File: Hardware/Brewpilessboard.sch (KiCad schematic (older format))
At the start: 10 parts, among them J1 Conn_01x01_Female, J2 Conn_01x01_Female, K1 2channelrelay, U1 ESP32_DevKit_V1_DOIT, U2 DS18B20, U3 DS18B20

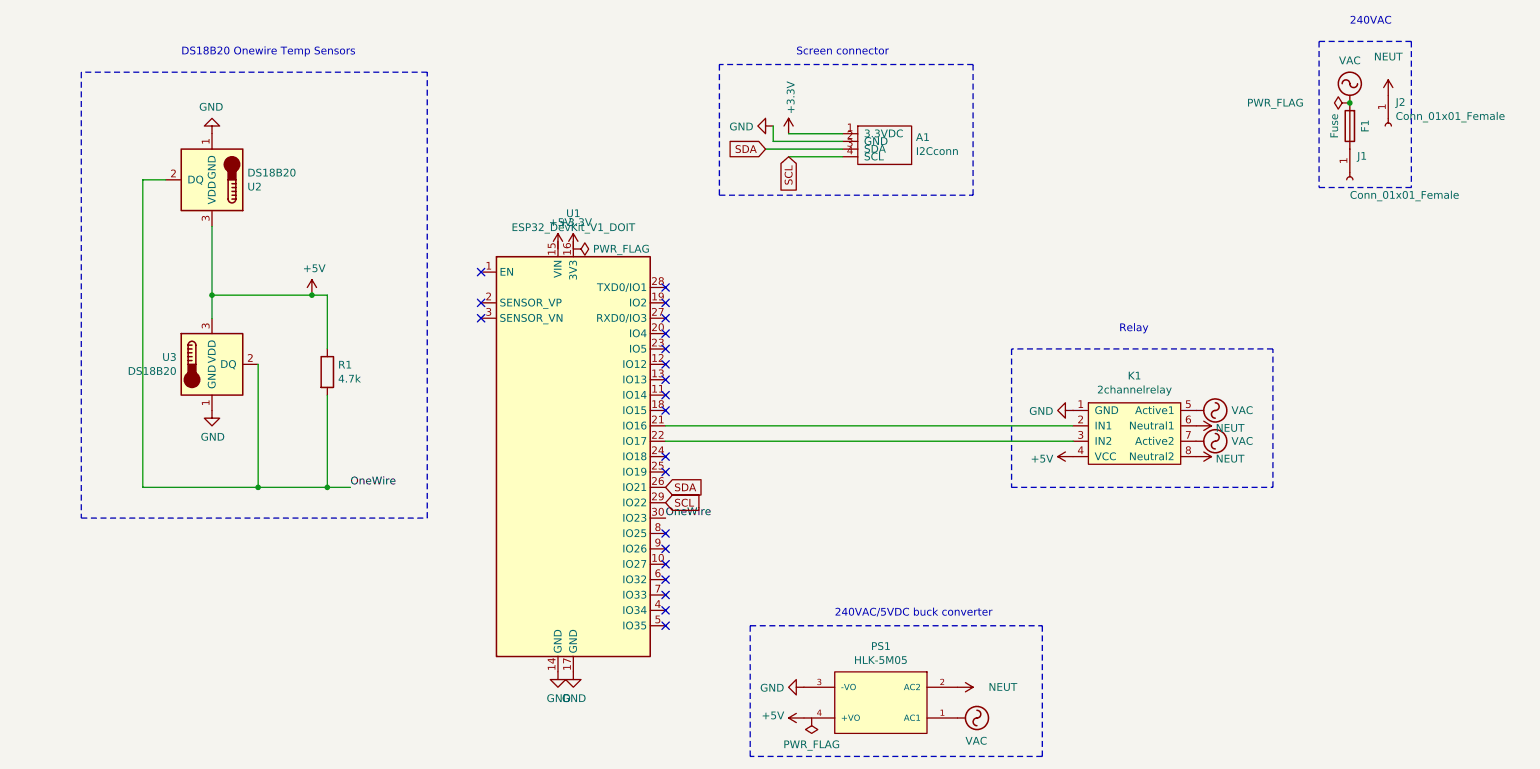
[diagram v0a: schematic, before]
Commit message: Further changes
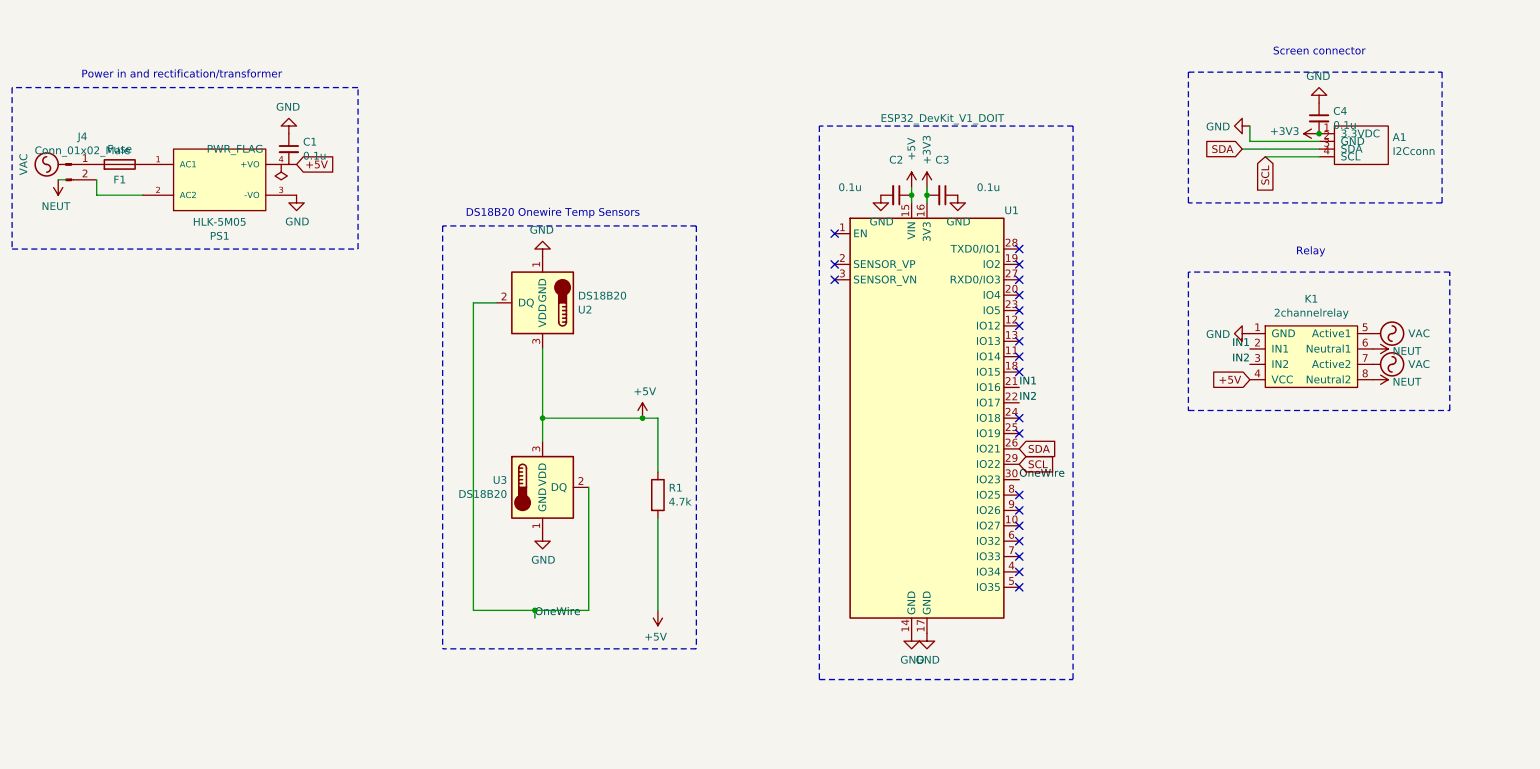
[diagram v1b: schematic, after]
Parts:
- removed J1, J2: Conn_01x01_Female, Connector_PinHeader_2.54mm:PinHeader_1x01_P2.54mm_Vertical, symbol Connector:Conn_01x01_Female
- added C1, C2, C3, C4: 0.1u, Capacitor_SMD:C_1206_3216Metric_Pad1.42x1.75mm_HandSolder, symbol Device:C_Small
- added J4: Conn_01x02_Male, Connector_JST:JST_XH_B2B-XH-AM_1x02_P2.50mm_Vertical, symbol Connector:Conn_01x02_Male
- R1: footprint Resistor_THT:R_Axial_DIN0204_L3.6mm_D1.6mm_P7.62mm_Horizontal -> Resistor_SMD:R_1206_3216Metric_Pad1.42x1.75mm_HandSolder
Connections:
- net labels added: +3V3, IN1, IN2
- net labels removed: +3.3V
- wire segments 19 -> 23
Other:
- note added: "Power in and rectification/transformer"
- note removed: "240VAC"
- note removed: "240VAC/5VDC buck converter"
- moved on the sheet: A1, F1, K1, PS1, R1, U1, U2, U3
